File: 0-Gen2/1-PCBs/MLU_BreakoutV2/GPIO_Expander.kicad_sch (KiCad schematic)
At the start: 8 parts, among them U7 MCP23008-E_P

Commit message: [final pass] MLU breakout
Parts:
- JP10, JP8, JP9: footprint Jumper:SolderJumper-3_P1.3mm_Bridged2Bar12_RoundedPad1.0x1.5mm -> Connector_PinHeader_1.27mm:PinHeader_1x03_P1.27mm_Vertical
- U7: footprint Imported Footprints:MCP3008 -> ImportedV2:MCP3008
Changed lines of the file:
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@@
 			)
 		)
-		(property "Footprint" "Jumper:SolderJumper-3_P1.3mm_Bridged2Bar12_RoundedPad1.0x1.5mm"
+		(property "Footprint" "Connector_PinHeader_1.27mm:PinHeader_1x03_P1.27mm_Vertical"
 			(at 93.98 75.946 0)
 			(effects
@@
 			)
 		)
-		(property "Footprint" "Imported Footprints:MCP3008"
+		(property "Footprint" "ImportedV2:MCP3008"
 			(at 163.322 92.71 0)
 			(effects
@@
 			)
 		)
-		(property "Footprint" "Jumper:SolderJumper-3_P1.3mm_Bridged2Bar12_RoundedPad1.0x1.5mm"
+		(property "Footprint" "Connector_PinHeader_1.27mm:PinHeader_1x03_P1.27mm_Vertical"
 			(at 75.438 83.82 0)
 			(effects
@@
 			)
 		)
-		(property "Footprint" "Jumper:SolderJumper-3_P1.3mm_Bridged2Bar12_RoundedPad1.0x1.5mm"
+		(property "Footprint" "Connector_PinHeader_1.27mm:PinHeader_1x03_P1.27mm_Vertical"
 			(at 111.76 111.252 0)
 			(effects

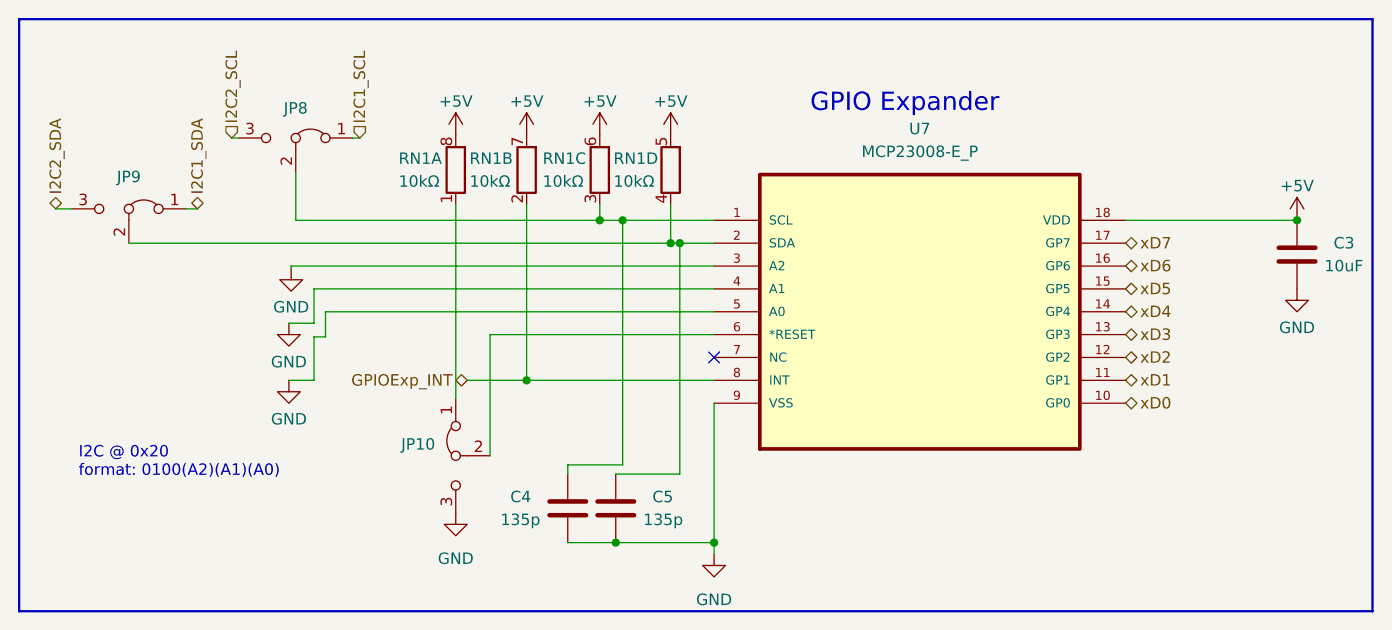
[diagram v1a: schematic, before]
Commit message: before restructure
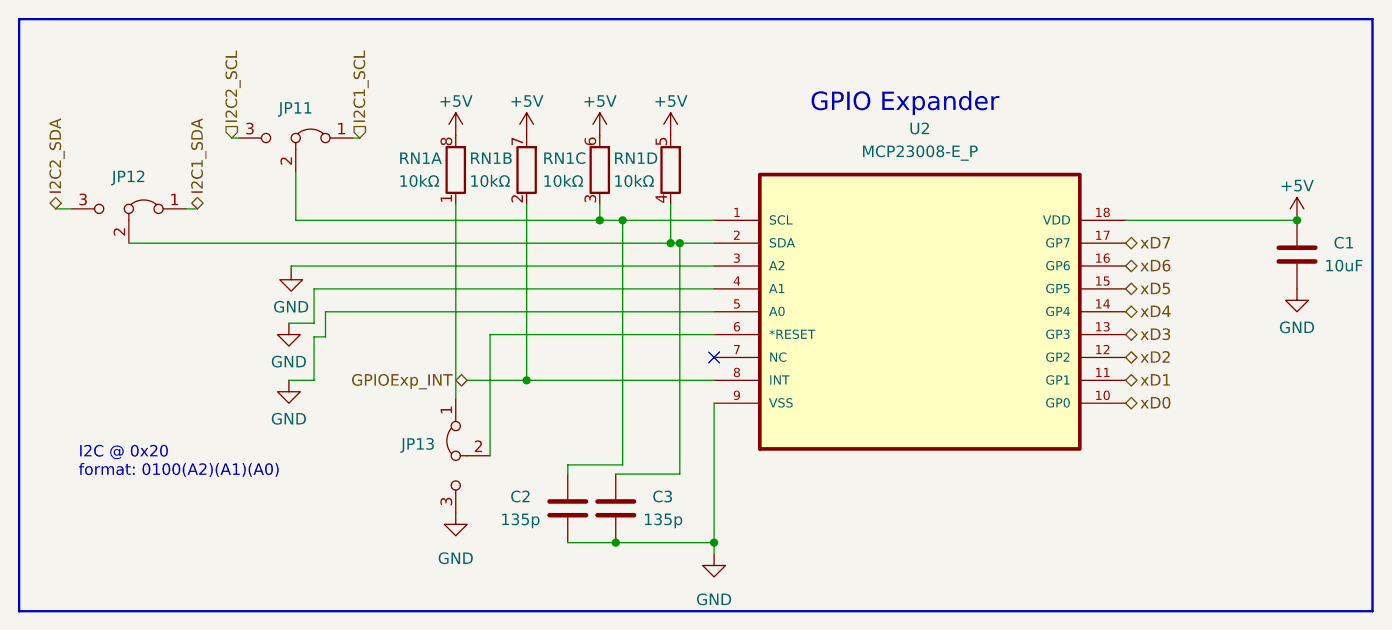
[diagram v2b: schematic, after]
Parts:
- renumbered C3 to C1, C4 to C2, C5 to C3, JP8 to JP11, JP9 to JP12, JP10 to JP13, U7 to U2
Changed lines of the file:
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@@
 		(dnp no)
 		(fields_autoplaced yes)
-		(property "Reference" "JP8"
+		(property "Reference" "JP11"
 			(at 93.98 72.644 0)
 			(effects
@@
 			(project "MLU_BreakoutV2"
 				(path "/55121ba7-5d22-4fe3-93aa-7f76d75b410c/ff819628-ab19-4c4a-a87c-3aa1c78e0ae1"
-					(reference "JP8")
+					(reference "JP11")
 					(unit 1)
 				)
@@
 		(on_board yes)
 		(dnp no)
-		(property "Reference" "C4"
+		(property "Reference" "C2"
 			(at 120.142 115.8239 0)
 			(effects
@@
 			(project "MLU_BreakoutV2"
 				(path "/55121ba7-5d22-4fe3-93aa-7f76d75b410c/ff819628-ab19-4c4a-a87c-3aa1c78e0ae1"
-					(reference "C4")
+					(reference "C2")
 					(unit 1)
 				)
@@
 		(on_board yes)
 		(dnp no)
-		(property "Reference" "#PWR0141"
+		(property "Reference" "#PWR090"
 			(at 205.232 88.9 0)
 			(effects
@@
 			(project "MLU_BreakoutV2"
 				(path "/55121ba7-5d22-4fe3-93aa-7f76d75b410c/ff819628-ab19-4c4a-a87c-3aa1c78e0ae1"
-					(reference "#PWR0141")
+					(reference "#PWR090")
 					(unit 1)
 				)
@@
 		(dnp no)
 		(fields_autoplaced yes)
-		(property "Reference" "#PWR0146"
+		(property "Reference" "#PWR095"
 			(at 111.76 123.952 0)
 			(effects
@@
 			(project "MLU_BreakoutV2"
 				(path "/55121ba7-5d22-4fe3-93aa-7f76d75b410c/ff819628-ab19-4c4a-a87c-3aa1c78e0ae1"
-					(reference "#PWR0146")
+					(reference "#PWR095")
 					(unit 1)
 				)
@@
 		(on_board yes)
 		(dnp no)
-		(property "Reference" "#PWR0137"
+		(property "Reference" "#PWR086"
 			(at 111.76 79.502 0)
 			(effects
@@
 			(project "MLU_BreakoutV2"
 				(path "/55121ba7-5d22-4fe3-93aa-7f76d75b410c/ff819628-ab19-4c4a-a87c-3aa1c78e0ae1"
-					(reference "#PWR0137")
+					(reference "#PWR086")
 					(unit 1)
 				)
@@
 		(dnp no)
 		(fields_autoplaced yes)
-		(property "Reference" "#PWR0143"
+		(property "Reference" "#PWR092"
 			(at 205.232 99.06 0)
 			(effects
@@
 			(project "MLU_BreakoutV2"
 				(path "/55121ba7-5d22-4fe3-93aa-7f76d75b410c/ff819628-ab19-4c4a-a87c-3aa1c78e0ae1"
-					(reference "#PWR0143")
+					(reference "#PWR092")
 					(unit 1)
 				)
@@
 		(dnp no)
 		(fields_autoplaced yes)
-		(property "Reference" "#PWR0144"
+		(property "Reference" "#PWR093"
 			(at 93.218 102.87 0)
 			(effects
@@
 			(project "MLU_BreakoutV2"
 				(path "/55121ba7-5d22-4fe3-93aa-7f76d75b410c/ff819628-ab19-4c4a-a87c-3aa1c78e0ae1"
-					(reference "#PWR0144")
+					(reference "#PWR093")
 					(unit 1)
 				)
@@
 		(dnp no)
 		(fields_autoplaced yes)
-		(property "Reference" "#PWR0145"
+		(property "Reference" "#PWR094"
 			(at 93.218 109.22 0)
 			(effects
@@
 			(project "MLU_BreakoutV2"
 				(path "/55121ba7-5d22-4fe3-93aa-7f76d75b410c/ff819628-ab19-4c4a-a87c-3aa1c78e0ae1"
-					(reference "#PWR0145")
+					(reference "#PWR094")
 					(unit 1)
 				)
@@
 		(on_board yes)
 		(dnp no)
-		(property "Reference" "C5"
+		(property "Reference" "C3"
 			(at 133.604 115.8239 0)
 			(effects
@@
 			(project "MLU_BreakoutV2"
 				(path "/55121ba7-5d22-4fe3-93aa-7f76d75b410c/ff819628-ab19-4c4a-a87c-3aa1c78e0ae1"
-					(reference "C5")
+					(reference "C3")
 					(unit 1)
 				)
@@
 		(on_board yes)
 		(dnp no)
-		(property "Reference" "#PWR0139"
+		(property "Reference" "#PWR088"
 			(at 127.762 79.502 0)
 			(effects
@@
 			(project "MLU_BreakoutV2"
 				(path "/55121ba7-5d22-4fe3-93aa-7f76d75b410c/ff819628-ab19-4c4a-a87c-3aa1c78e0ae1"
-					(reference "#PWR0139")
+					(reference "#PWR088")
 					(unit 1)
 				)
@@
 		(dnp no)
 		(fields_autoplaced yes)
-		(property "Reference" "U7"
+		(property "Reference" "U2"
 			(at 163.322 74.93 0)
 			(effects
@@
 			(project "MLU_BreakoutV2"
 				(path "/55121ba7-5d22-4fe3-93aa-7f76d75b410c/ff819628-ab19-4c4a-a87c-3aa1c78e0ae1"
-					(reference "U7")
+					(reference "U2")
 					(unit 1)
 				)
@@
 		(dnp no)
 		(fields_autoplaced yes)
-		(property "Reference" "#PWR0147"
+		(property "Reference" "#PWR096"
 			(at 140.462 128.524 0)
 			(effects
@@
 			(project "MLU_BreakoutV2"
 				(path "/55121ba7-5d22-4fe3-93aa-7f76d75b410c/ff819628-ab19-4c4a-a87c-3aa1c78e0ae1"
-					(reference "#PWR0147")
+					(reference "#PWR096")
 					(unit 1)
 				)
@@
 		(on_board yes)
 		(dnp no)
-		(property "Reference" "#PWR0140"
+		(property "Reference" "#PWR089"
 			(at 135.636 79.502 0)
 			(effects
@@
 			(project "MLU_BreakoutV2"
 				(path "/55121ba7-5d22-4fe3-93aa-7f76d75b410c/ff819628-ab19-4c4a-a87c-3aa1c78e0ae1"
-					(reference "#PWR0140")
+					(reference "#PWR089")
 					(unit 1)
 				)
@@
 		(dnp no)
 		(fields_autoplaced yes)
-		(property "Reference" "#PWR0142"
+		(property "Reference" "#PWR091"
 			(at 93.472 96.774 0)
 			(effects
@@
 			(project "MLU_BreakoutV2"
 				(path "/55121ba7-5d22-4fe3-93aa-7f76d75b410c/ff819628-ab19-4c4a-a87c-3aa1c78e0ae1"
-					(reference "#PWR0142")
+					(reference "#PWR091")
 					(unit 1)
 				)
@@
 		(on_board yes)
 		(dnp no)
-		(property "Reference" "C3"
+		(property "Reference" "C1"
 			(at 209.296 87.6299 0)
 			(effects
@@
 			(project "MLU_BreakoutV2"
 				(path "/55121ba7-5d22-4fe3-93aa-7f76d75b410c/ff819628-ab19-4c4a-a87c-3aa1c78e0ae1"
-					(reference "C3")
+					(reference "C1")
 					(unit 1)
 				)
@@
 		(dnp no)
 		(fields_autoplaced yes)
-		(property "Reference" "JP9"
+		(property "Reference" "JP12"
 			(at 75.438 80.264 0)
 			(effects
@@
 			(project "MLU_BreakoutV2"
 				(path "/55121ba7-5d22-4fe3-93aa-7f76d75b410c/ff819628-ab19-4c4a-a87c-3aa1c78e0ae1"
-					(reference "JP9")
+					(reference "JP12")
 					(unit 1)
 				)
@@
 		(on_board yes)
 		(dnp no)
-		(property "Reference" "#PWR0138"
+		(property "Reference" "#PWR087"
 			(at 119.634 79.502 0)
 			(effects
@@
 			(project "MLU_BreakoutV2"
 				(path "/55121ba7-5d22-4fe3-93aa-7f76d75b410c/ff819628-ab19-4c4a-a87c-3aa1c78e0ae1"
-					(reference "#PWR0138")
+					(reference "#PWR087")
 					(unit 1)
 				)
@@
 		(dnp no)
 		(fields_autoplaced yes)
-		(property "Reference" "JP10"
+		(property "Reference" "JP13"
 			(at 109.474 109.9819 90)
 			(effects
@@
 			(project "MLU_BreakoutV2"
 				(path "/55121ba7-5d22-4fe3-93aa-7f76d75b410c/ff819628-ab19-4c4a-a87c-3aa1c78e0ae1"
-					(reference "JP10")
+					(reference "JP13")
 					(unit 1)
 				)
